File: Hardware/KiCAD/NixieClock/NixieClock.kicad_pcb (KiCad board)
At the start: 2 copper layers, 232.9 x 67.3 mm, 37 parts, among them IC1 , IC2 , IC3 , IC4 , IC5 , IC6 , IC7 , IC8 , IC9 

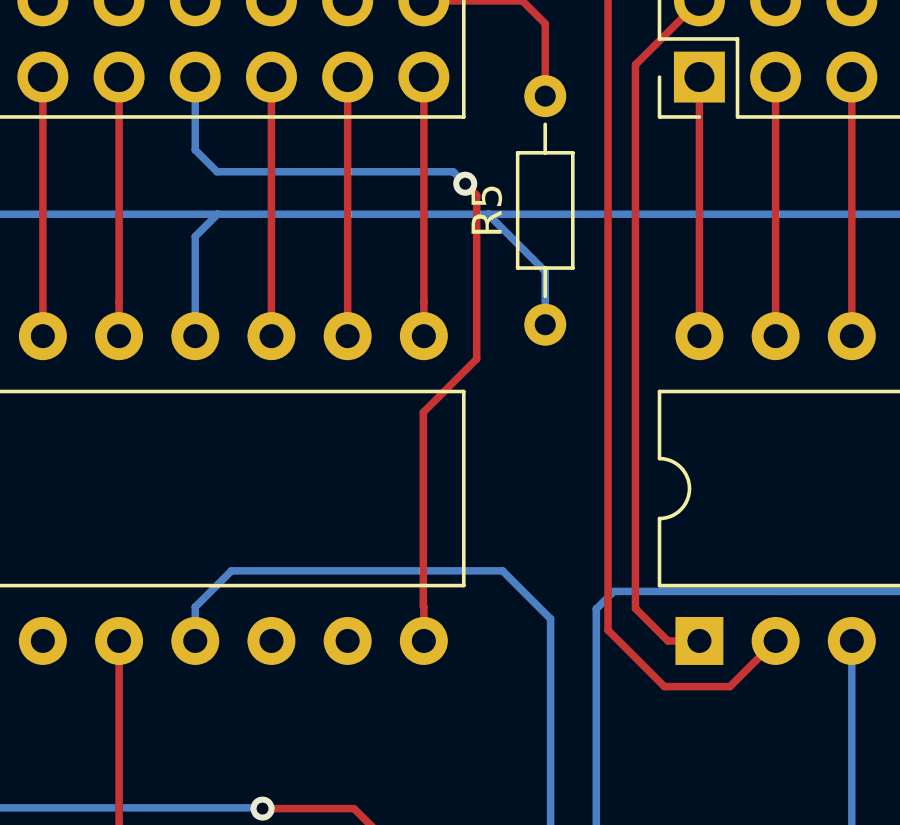
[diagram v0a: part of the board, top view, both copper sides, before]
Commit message: progress
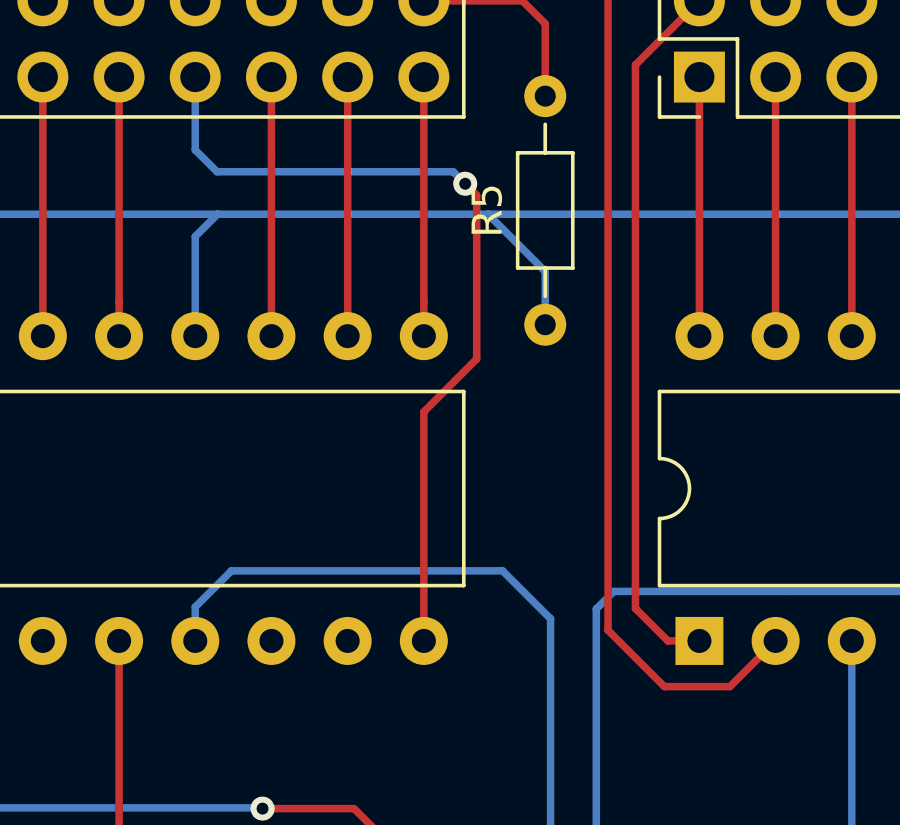
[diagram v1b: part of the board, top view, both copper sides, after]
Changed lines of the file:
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@@
     (thickness 1.6)
     (drawings 16)
-    (tracks 819)
+    (tracks 816)
     (zones 0)
     (modules 37)
@@
       (drillshape 0)
       (scaleselection 1)
-      (outputdirectory ""))
+      (outputdirectory "../Gerbers/"))
   )
   (net 0 "")
@@
   (segment (start 143.637 89.281) (end 142.68 88.324) (width 0.25) (layer B.Cu) (net 0))
   (segment (start 151.638 89.789) (end 151.13 89.281) (width 0.25) (layer B.Cu) (net 0))
-  (segment (start 123.335 104.02463) (end 123.317 104.00663) (width 0.25) (layer F.Cu) (net 0))
-  (segment (start 123.335 105.156) (end 123.335 104.02463) (width 0.25) (layer F.Cu) (net 0))
-  (segment (start 123.317 104.00663) (end 123.317 97.536) (width 0.25) (layer F.Cu) (net 0))
-  (segment (start 123.317 97.536) (end 125.095 95.758) (width 0.25) (layer F.Cu) (net 0))
-  (segment (start 125.095 95.758) (end 125.095 90.551) (width 0.25) (layer F.Cu) (net 0))
-  (segment (start 125.095 90.551) (end 125.095 90.297) (width 0.25) (layer F.Cu) (net 0))
   (via (at 124.714 89.916) (size 0.8) (drill 0.4) (layers F.Cu B.Cu) (net 0))
-  (segment (start 125.095 90.297) (end 124.714 89.916) (width 0.25) (layer F.Cu) (net 0))
   (segment (start 124.314001 89.516001) (end 116.440001 89.516001) (width 0.25) (layer B.Cu) (net 0))
   (segment (start 124.714 89.916) (end 124.314001 89.516001) (width 0.25) (layer B.Cu) (net 0))
@@
   (segment (start 221.996 72.39) (end 224.282 74.676) (width 0.25) (layer F.Cu) (net 0))
   (segment (start 200.025 72.39) (end 221.996 72.39) (width 0.25) (layer F.Cu) (net 0))
+  (segment (start 123.335 97.518) (end 123.335 105.156) (width 0.25) (layer F.Cu) (net 0))
+  (segment (start 125.095 95.758) (end 123.335 97.518) (width 0.25) (layer F.Cu) (net 0))
+  (segment (start 125.095 90.297) (end 125.095 95.758) (width 0.25) (layer F.Cu) (net 0))
+  (segment (start 124.714 89.916) (end 125.095 90.297) (width 0.25) (layer F.Cu) (net 0))
 )
